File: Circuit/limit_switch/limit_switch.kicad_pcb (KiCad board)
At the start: 2 copper layers, 25.4 x 48.5 mm, 21 parts

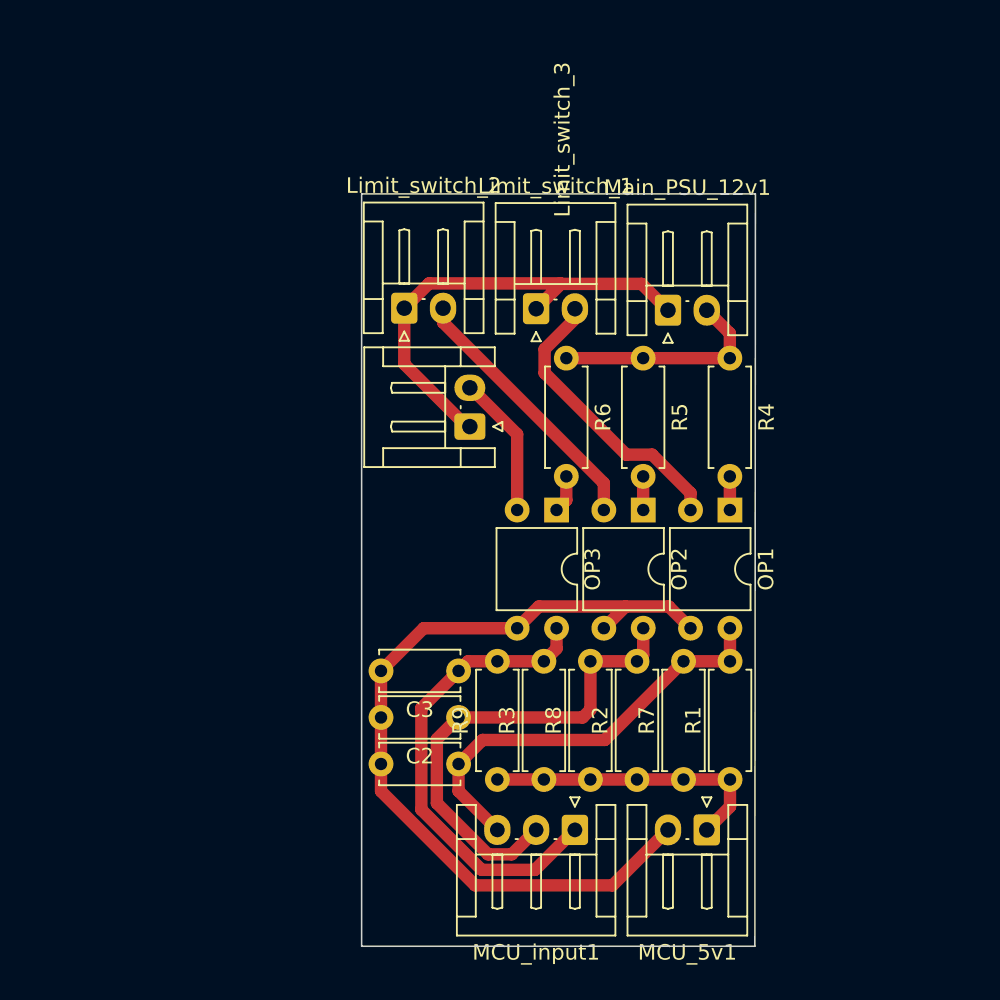
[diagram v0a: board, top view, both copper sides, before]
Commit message: further development in esp32-cam
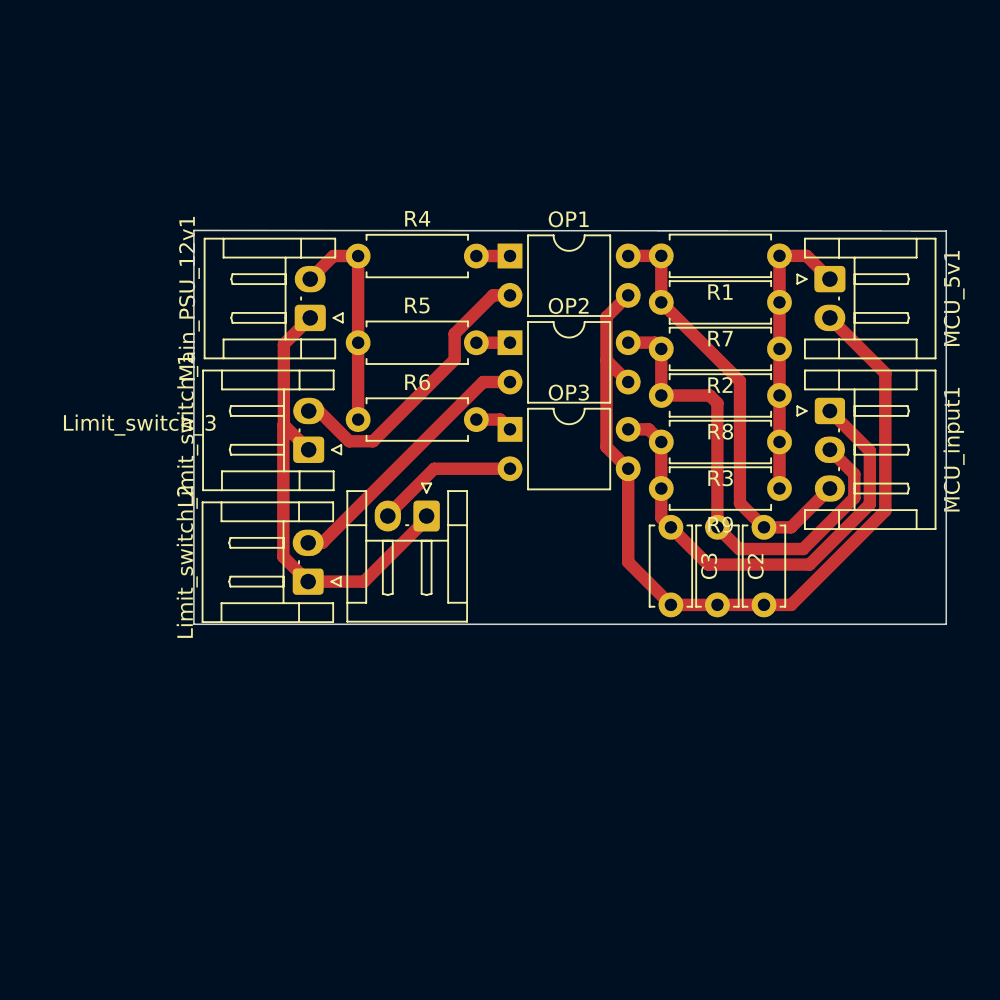
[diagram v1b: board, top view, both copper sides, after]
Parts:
- moved MCU_5v1 36.4 mm to (195.9, 86.5), turned to -90 degrees
- moved R1 33.9 mm to (192.6, 85.0), turned to 180 degrees
- moved MCU_input1 31.6 mm to (195.9, 95.0), turned to -90 degrees
- moved R7 31.4 mm to (192.6, 88.0), turned to 180 degrees
- moved R2 29.2 mm to (192.6, 91.0), turned to 180 degrees
- moved R8 27.6 mm to (192.6, 94.0), turned to 180 degrees
- moved R3 26.5 mm to (192.6, 97.0), turned to 180 degrees
- moved R9 26.1 mm to (192.6, 100.0), turned to 180 degrees
- moved C1 24.9 mm to (191.6, 102.5), turned to -90 degrees
- moved R4 24.8 mm to (165.5, 85.0), turned to 0 degrees
- moved Main_PSU_12v1 23.1 mm to (162.4, 89.0), turned to 90 degrees
- moved OP1 21.7 mm to (175.2, 85.0), turned to 0 degrees
- moved C2 20.7 mm to (188.6, 102.5), turned to -90 degrees
- moved Limit_switch_2 18.7 mm to (162.2, 106.0), turned to 90 degrees
- moved R5 18.4 mm to (165.5, 90.6), turned to 0 degrees
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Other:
- board size 25.4 x 48.5 mm -> 48.5 x 25.4 mm
